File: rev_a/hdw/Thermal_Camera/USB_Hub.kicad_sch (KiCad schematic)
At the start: 1 part

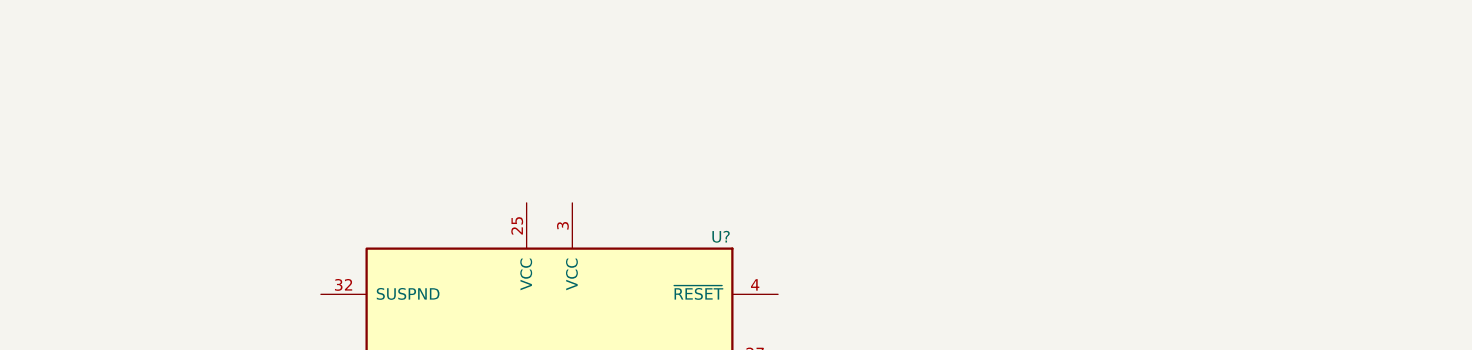
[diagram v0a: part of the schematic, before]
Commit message: duplicated telemetry for all rails, added random tweaks to logic levels of signals
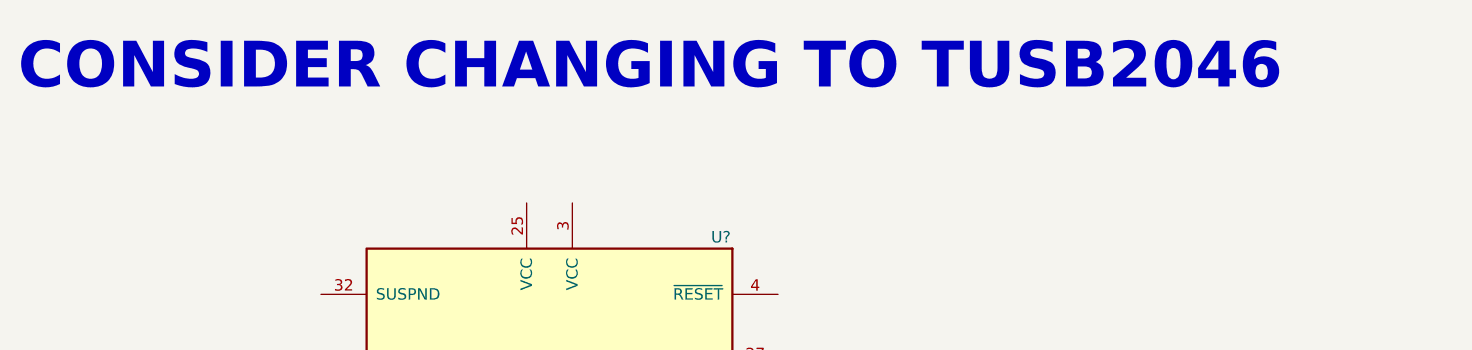
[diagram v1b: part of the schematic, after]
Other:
- note added: "CONSIDER CHANGING TO TUSB2046"
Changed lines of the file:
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@@
     (company "Drew Maatman and Michael Laffin")
+  )
+  (text "CONSIDER CHANGING TO TUSB2046" (at 72.39 38.735 0)
+    (effects (font (face "Courier New") (size 5.08 5.08) (thickness 1.016) bold (color 194 0 0 1)) (justify left bottom))
   )
   (symbol (lib_id "Interface_USB:TUSB2036") (at 131.445 91.44 0) (mirror y) (unit 1)
